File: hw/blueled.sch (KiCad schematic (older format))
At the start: 53 parts, among them J1 Barrel_Jack, J2 LED Strip, J3 ICSP, J4 Screw_Terminal_01x02, Q1 Q_PMOS_SDG, Q2 Q_PNP_EBC, SW2 PUSH, U1 ATmega328P-AU, U2 HC-05, U3 AMS1117-3.3, U4 AT25SF081, X1 CSTCE

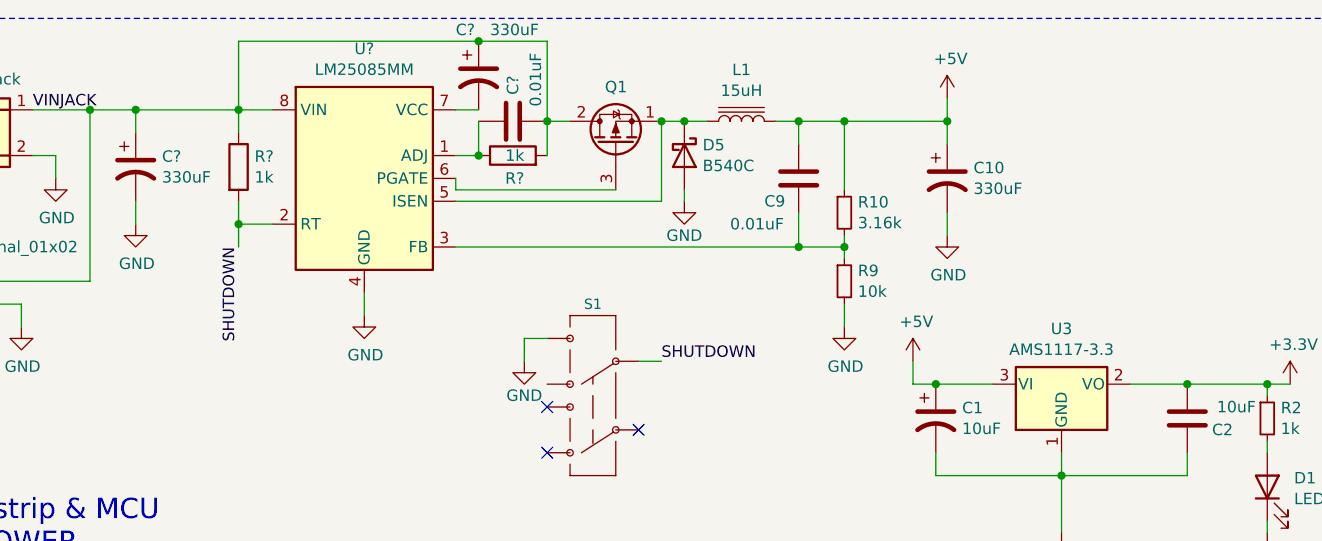
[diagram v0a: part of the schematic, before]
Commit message: add: missing comments (more to go)
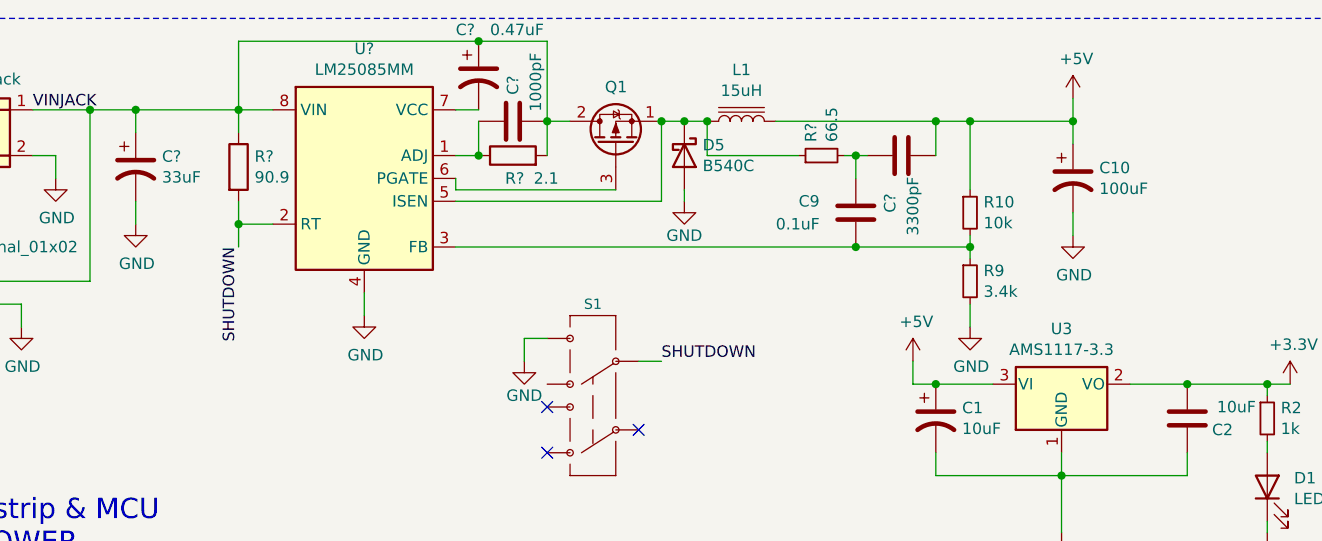
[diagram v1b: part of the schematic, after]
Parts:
- added C?: 3300pF, symbol Device:C
- added R?: 66.5, symbol Device:R_Small
- C10: value 330uF -> 100uF; footprint Capacitor_Tantalum_SMD:CP_EIA-3216-18_Kemet-A_Pad1.58x1.35mm_HandSolder -> (none)
- C9: value 0.01uF -> 0.1uF; footprint Capacitor_SMD:C_0805_2012Metric_Pad1.15x1.40mm_HandSolder -> (none)
- C?: value 330uF -> 33uF; footprint Capacitor_Tantalum_SMD:CP_EIA-3216-18_Kemet-A_Pad1.58x1.35mm_HandSolder -> (none)
- C?: value 330uF -> 0.47uF; footprint Capacitor_Tantalum_SMD:CP_EIA-3216-18_Kemet-A_Pad1.58x1.35mm_HandSolder -> (none)
- C?: value 0.01uF -> 1000pF; footprint Capacitor_SMD:C_0805_2012Metric_Pad1.15x1.40mm_HandSolder -> (none)
- R10: value 3.16k -> 10k; footprint Resistor_SMD:R_0805_2012Metric_Pad1.15x1.40mm_HandSolder -> (none)
- R9: value 10k -> 3.4k; footprint Resistor_SMD:R_0805_2012Metric_Pad1.15x1.40mm_HandSolder -> (none)
- R?: value 1k -> 90.9
- R?: value 1k -> 2.1; footprint Resistor_SMD:R_0805_2012Metric_Pad1.15x1.40mm_HandSolder -> (none)
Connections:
- net +5V: now also C?.2; no longer C9.1
- net at D5.1 (K), L1.1, Q1.1 (S)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: now also R?.1
- new net: C9.1, C?.1, R?.2
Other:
- moved on the sheet: C10, C9, R10, R9
